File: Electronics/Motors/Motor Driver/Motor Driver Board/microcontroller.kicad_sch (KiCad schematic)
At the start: 61 parts, among them IC1 STM32H723ZGT6, IC2 TJA1057GT/3, IC3 ESDA6V1W5, IC4 ESDA6V1W5, J1 TYPE-C-31-M-12, J2 Screw_Terminal_01x02, J3 TC2030, SW1 SW_DIP_x02, U1 LSM6DS3, X1 25MHz_Clock, X2 32.768kHz_Clock

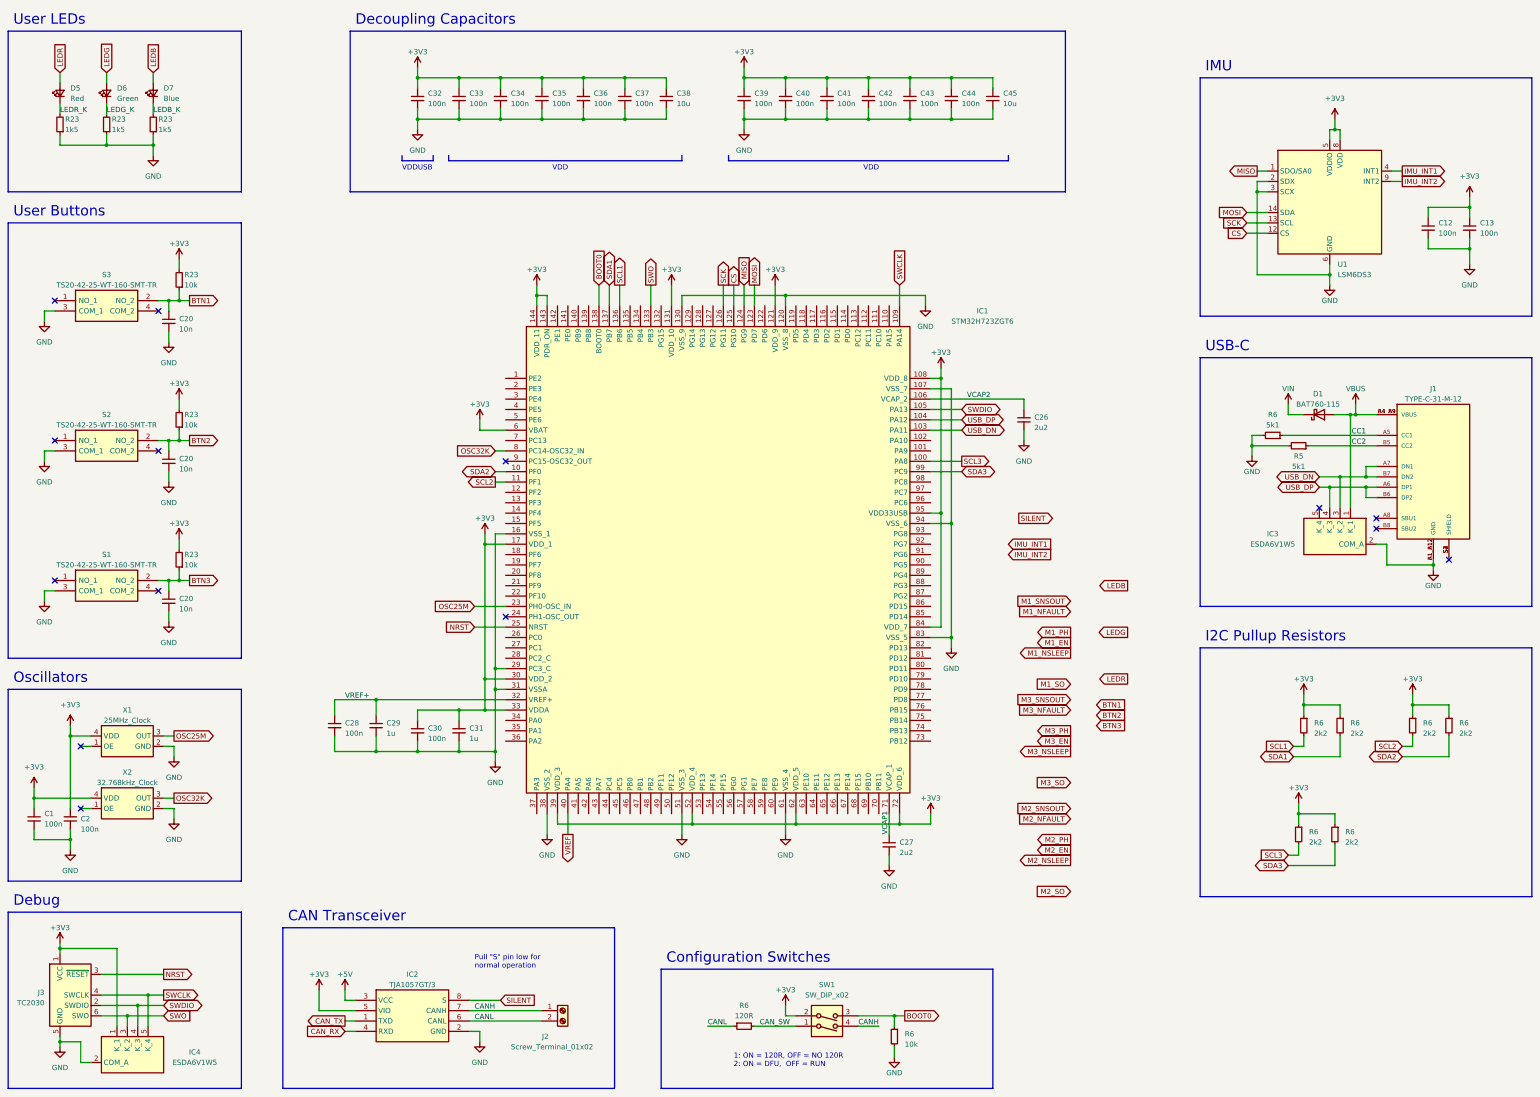
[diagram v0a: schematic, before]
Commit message: PCB Schematic progress
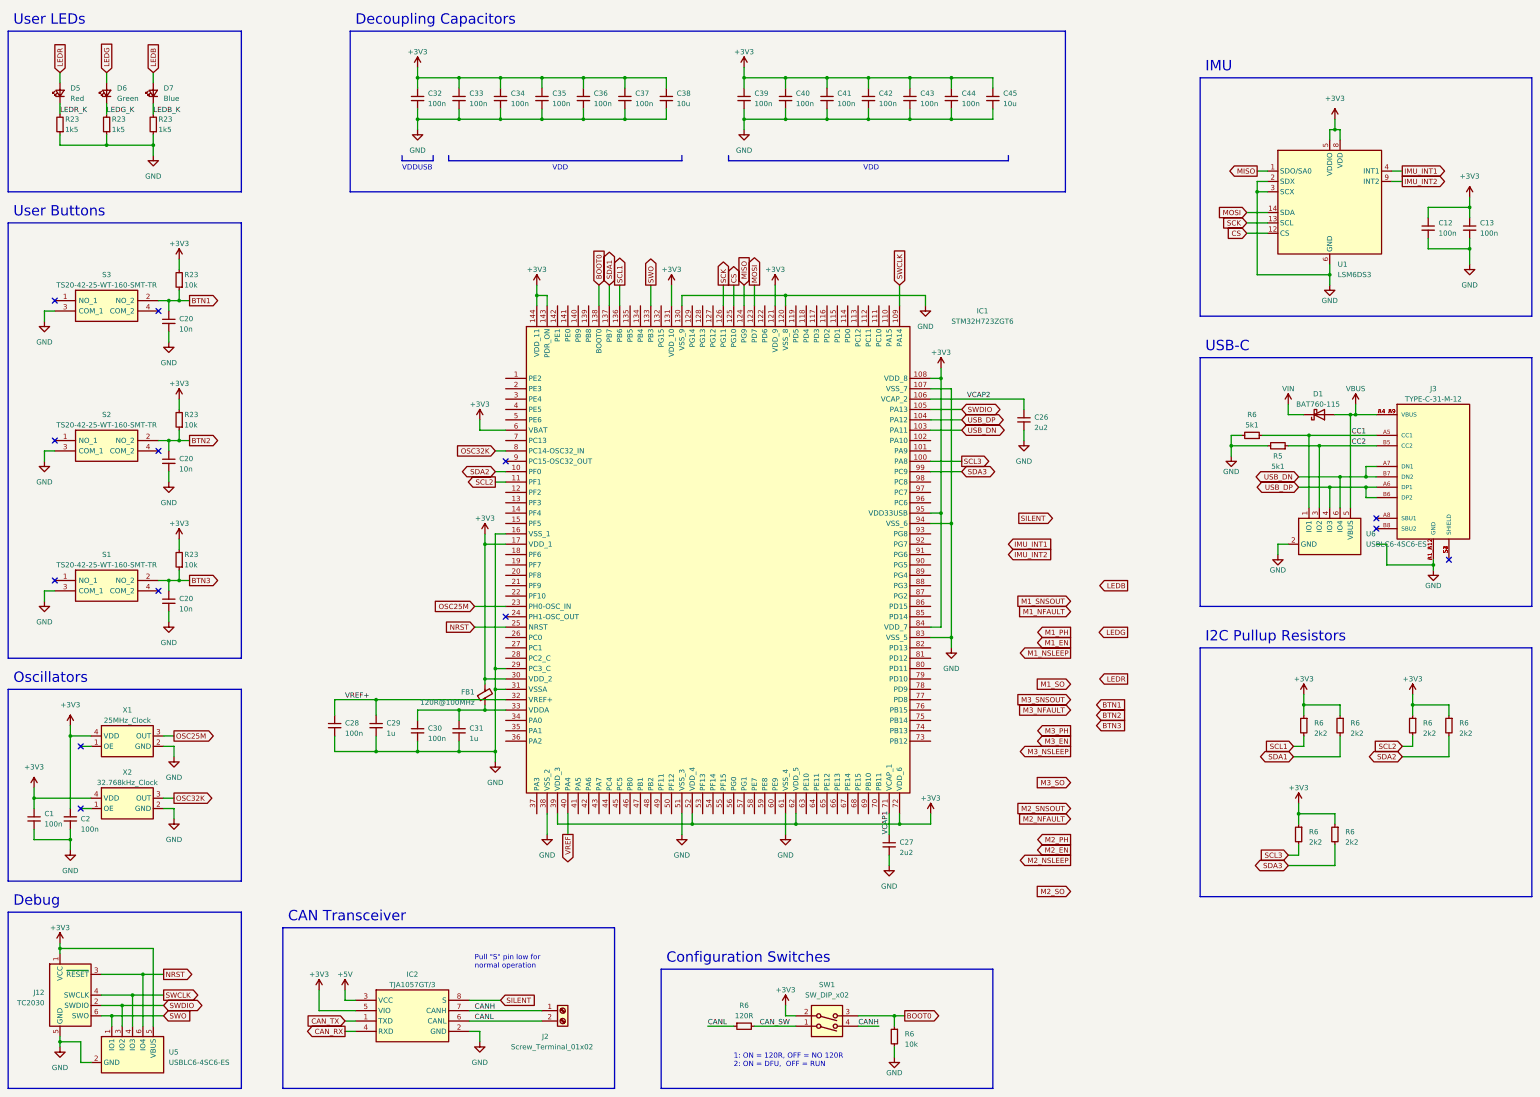
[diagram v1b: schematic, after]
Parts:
- removed IC3, IC4: ESDA6V1W5, SOT65P210X110-5N, symbol ESDA6V1W5:ESDA6V1W5
- removed J1: TYPE-C-31-M-12, MSL Footprints:HRO_TYPE-C-31-M-12, symbol TYPE-C-31-M-12:TYPE-C-31-M-12
- removed J3: TC2030, Connector:Tag-Connect_TC2030-IDC-FP_2x03_P1.27mm_Vertical, symbol Connector:Conn_ARM_SWD_TagConnect_TC2030
- added FB1: 120R@100MHz, Resistor_SMD:R_0402_1005Metric, symbol Device:FerriteBead_Small
- added J12: TC2030, Connector:Tag-Connect_TC2030-IDC-FP_2x03_P1.27mm_Vertical, symbol Connector:Conn_ARM_SWD_TagConnect_TC2030
- added J3: TYPE-C-31-M-12, MSL Footprints:HRO_TYPE-C-31-M-12, symbol TYPE-C-31-M-12:TYPE-C-31-M-12
- added U5, U6: USBLC6-4SC6-ES, Package_TO_SOT_SMD:SOT-23-6, symbol MSL_Symbols:USBLC6-4SC6-ES
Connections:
- net +3V3: now also FB1.2, J12.1 (VCC), U5.5 (VBUS); no longer C30.1, C31.1, IC1.33 (VDDA)
- net CC1: now also J3.A5 (CC1), U6.1 (IO1)
- net CC2: now also J3.B5 (CC2), U6.3 (IO2)
- net GND: now also J12.5 (GND), J3.A1_B12 (GND), J3.B1_A12 (GND), U5.2 (GND), U6.2 (GND)
- net NRST: now also J12.3 (~{RESET}), U5.6 (IO4)
- net SWCLK: now also J12.4 (SWCLK), U5.4 (IO3)
- net SWDIO: now also J12.2 (SWDIO), U5.3 (IO2)
- net SWO: now also J12.6 (SWO), U5.1 (IO1)
- net USB_DN: now also J3.A7 (DN1), J3.B7 (DN2), U6.6 (IO4)
- net USB_DP: now also J3.A6 (DP1), J3.B6 (DP2), U6.4 (IO3)
- net VBUS: now also J3.A4_B9 (VBUS), J3.B4_A9 (VBUS), U6.5 (VBUS)
- new net: C30.1, C31.1, FB1.1, IC1.33 (VDDA)
- new net: J3.S1 (SHIELD), J3.S2 (SHIELD), J3.S3 (SHIELD), J3.S4 (SHIELD)
- no-connect marks 14 -> 13
